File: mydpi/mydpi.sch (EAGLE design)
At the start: 26 parts, among them Q1 DMN3404L, U1 MEGA32U4-MU, U2 AP7381-33Y-13

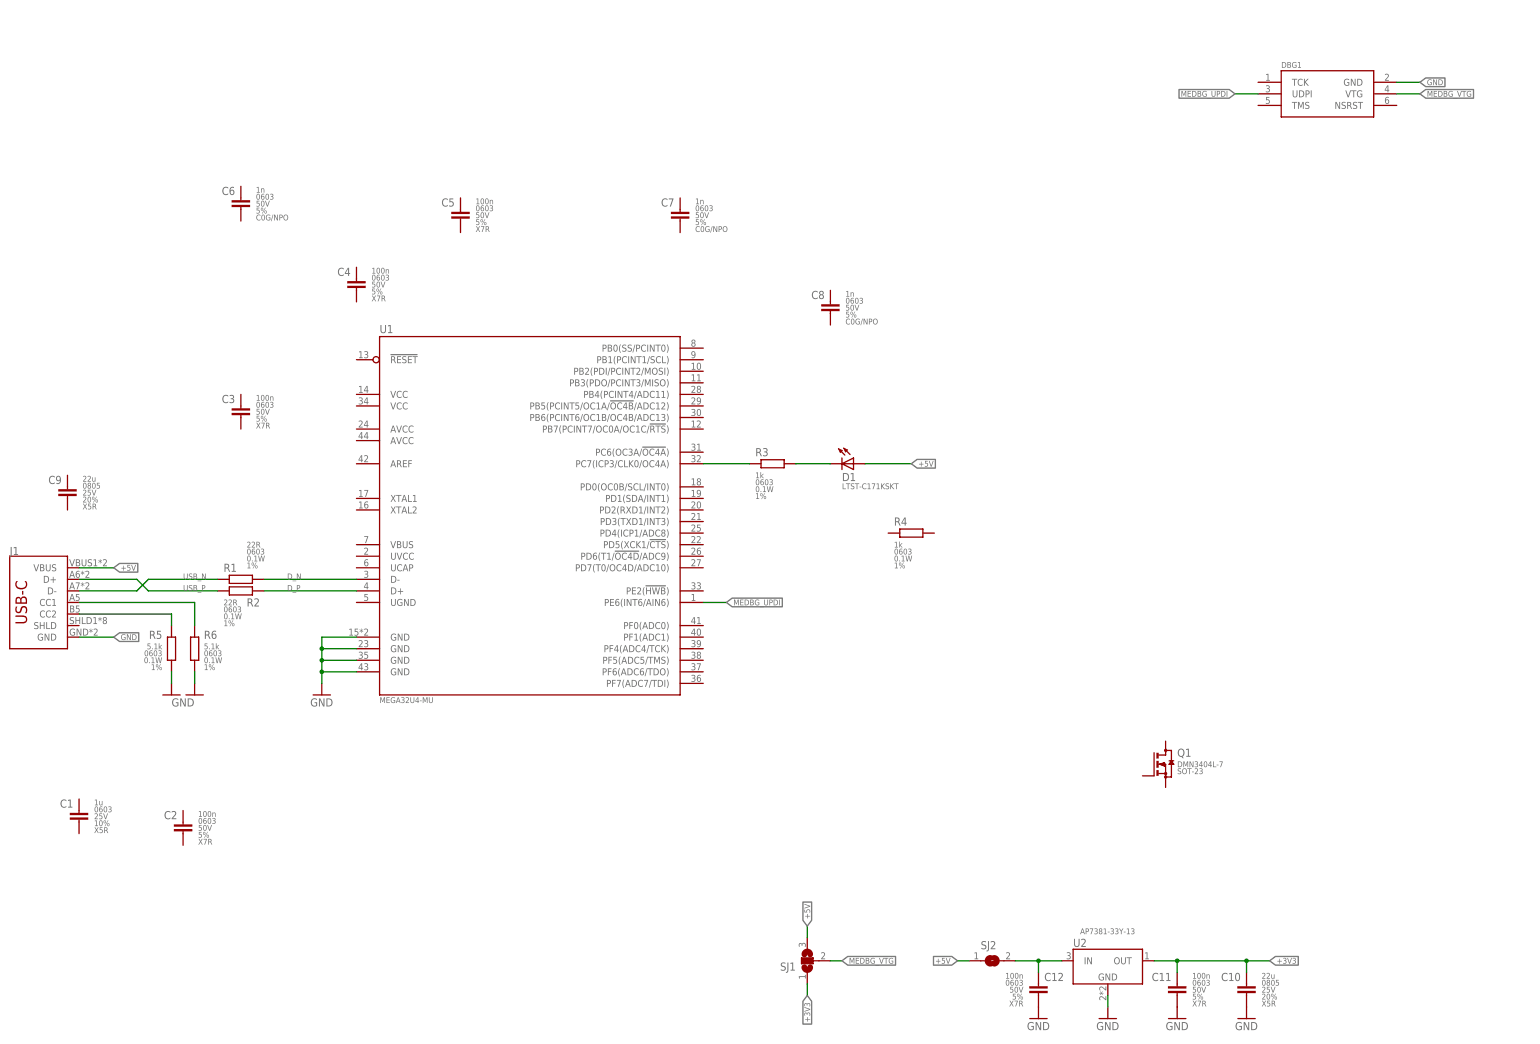
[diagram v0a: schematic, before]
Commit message: Placement LDO, Caps
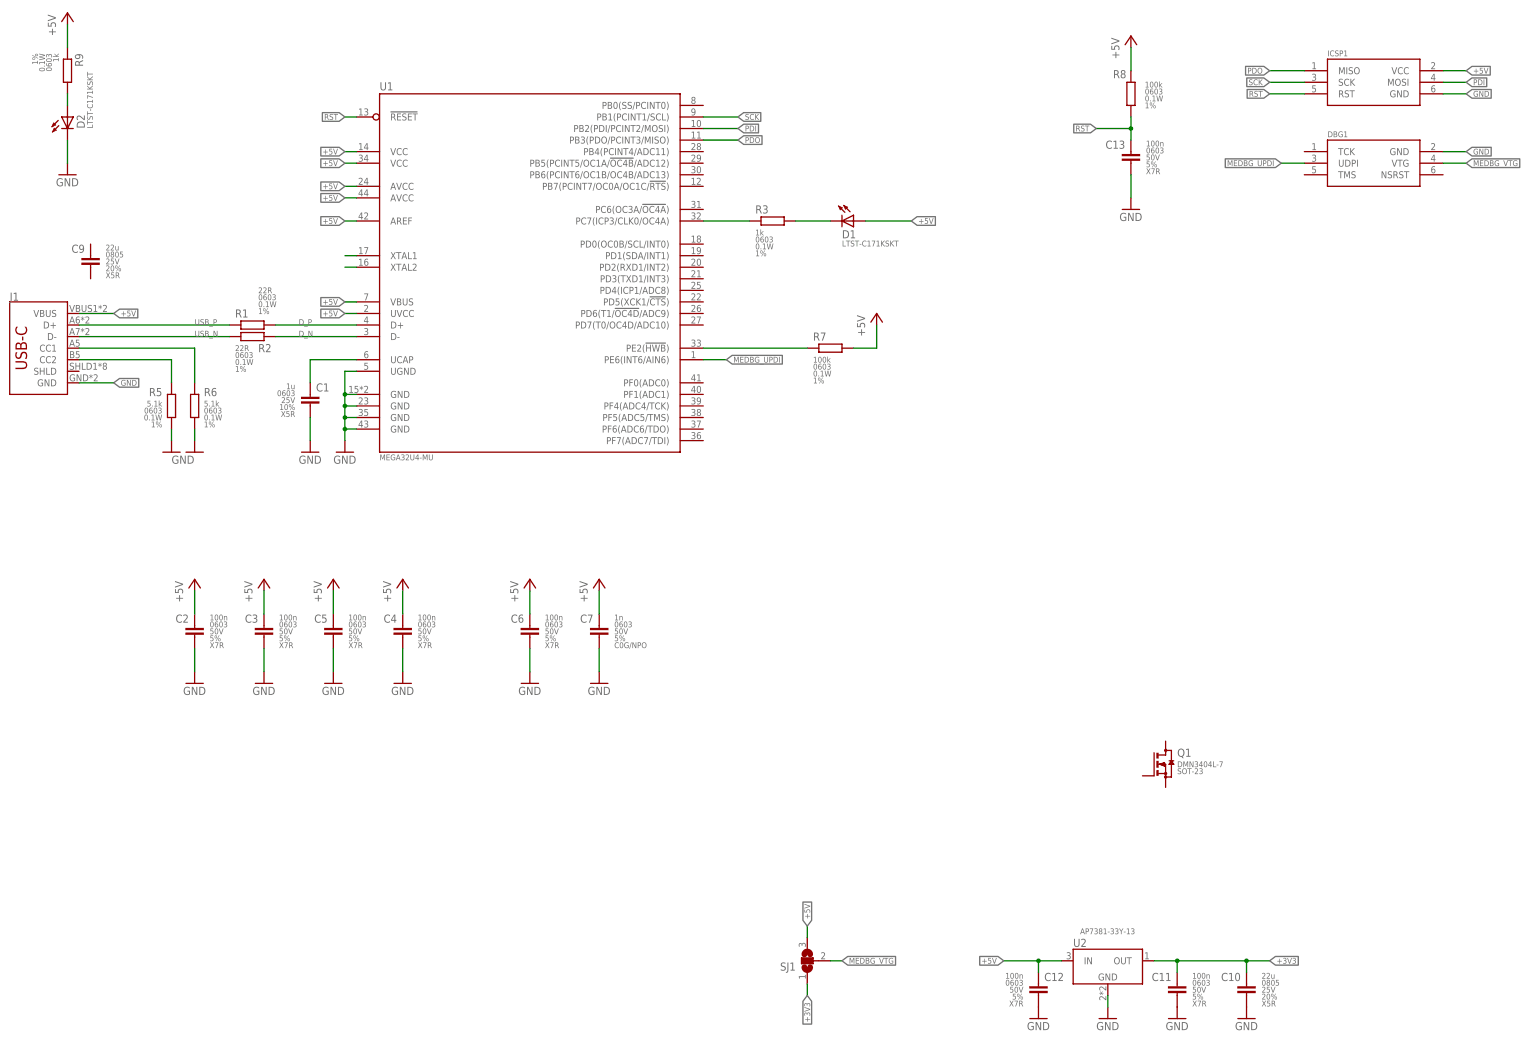
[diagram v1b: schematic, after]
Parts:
- removed C8: 1n, zaan-Capacitors:1NF-0603-50V-5%
- removed R4: 1k, zaan-Resistors:1KOHM-0603-1/10W-1%
- removed SJ2: (no value), jumper:SJ
- added C13: 100n, zaan-Capacitors:100NF-0603-50V-5%
- added D2: LTST-C171KSKT, zaan-Optoelectronics:LTST-C171KSKT
- added ICSP1: AVR-ISP-1.27MM, zaan-Connectors:AVR-ISP-1.27MM
- added R7, R8: 100k, zaan-Resistors:100KOHM-0603-1/10W-1%
- added R9: 1k, zaan-Resistors:1KOHM-0603-1/10W-1%
- C6: value 1n -> 100n; device zaan-Capacitors:1NF-0603-50V-5% -> zaan-Capacitors:100NF-0603-50V-5%
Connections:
- removed net N$4: C12.1, SJ2.2, U2.IN
- new net N$13: U1.XTAL1
- new net N$14: U1.XTAL2
- new net N$7: R7.1, U1.PE2(!HWB!)
- new net N$8: C1.1, U1.UCAP
- new net N$9: D2.A, R9.2
- new net PDI: ICSP1.MOSI, U1.PB2(PDI/PCINT2/MOSI)
- new net PDO: ICSP1.MISO, U1.PB3(PDO/PCINT3/MISO)
- new net RST: C13.1, ICSP1.RST, R8.1, U1.!RESET!
- new net SCK: ICSP1.SCK, U1.PB1(PCINT1/SCL)
- net +5V: now also C12.1, C2.1, C3.1, C4.1, C5.1, C6.1, C7.1, ICSP1.VCC, R7.2, R8.2, R9.1, U1.AREF, U1.AVCC@1, U1.AVCC@2, U1.UVCC, U1.VBUS, U1.VCC@1, U1.VCC@2, U2.IN; no longer SJ2.1
- net D_N: now also R2.2; no longer R1.2
- net D_P: now also R1.2; no longer R2.2
- net GND: now also C1.2, C13.2, C2.2, C3.2, C4.2, C5.2, C6.2, C7.2, D2.C, ICSP1.GND, U1.UGND
- net USB_N: now also R2.1; no longer R1.1
- net USB_P: now also R1.1; no longer R2.1
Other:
- moved on the sheet: C1, C2, C3, C4, C5, C6, C7, C9, D1, DBG1, J1, R1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
